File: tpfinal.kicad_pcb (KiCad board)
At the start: 2 copper layers, 108.1 x 81.5 mm, 17 parts, among them J1 220V, J2 1,5-30V 1,5A, SW2 SW_SPST, U1 LM317_TO-220

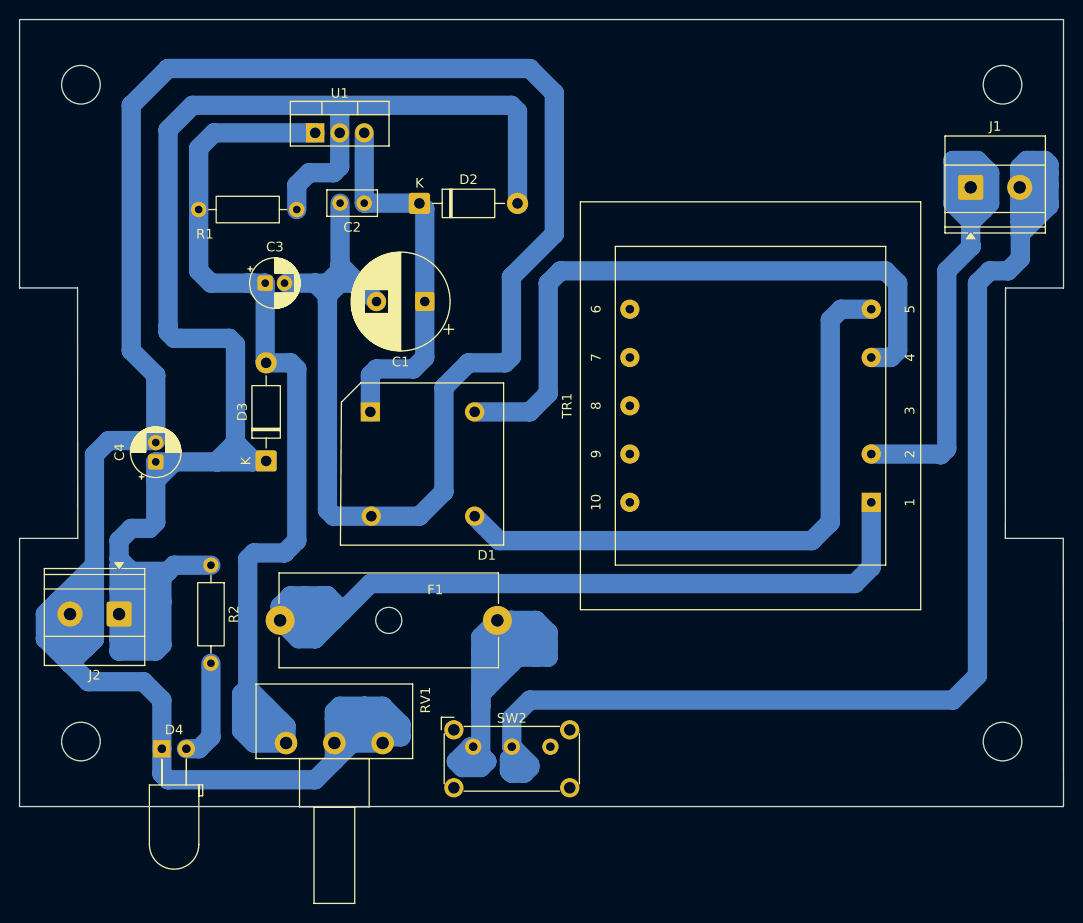
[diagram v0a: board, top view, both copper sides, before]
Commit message: Update
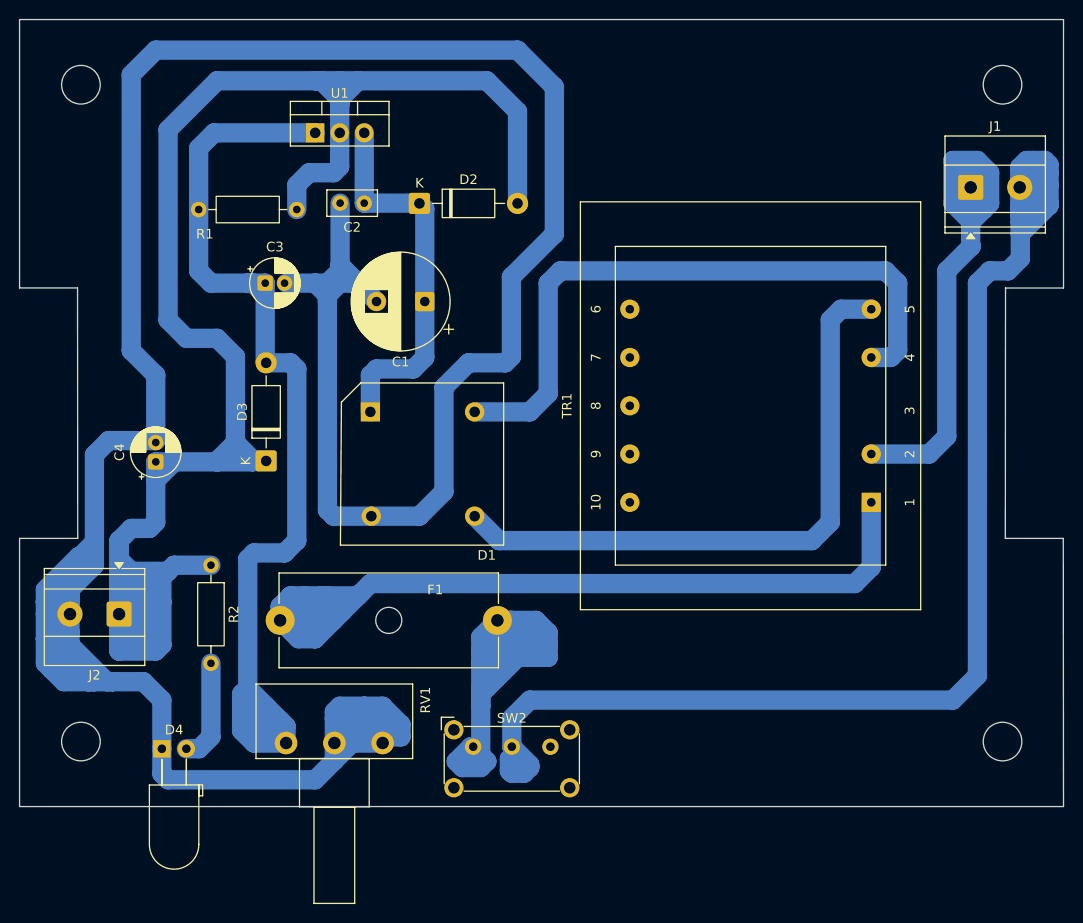
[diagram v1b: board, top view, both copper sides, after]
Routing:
- net +VDC: track 197.6 -> 218.6 mm
- net Net-(SW2-B): track 61.9 -> 74.3 mm
- net GND: track 348.6 -> 359.1 mm
- net Net-(F1-Pad2): track 102.5 -> 106.1 mm
- net Net-(J1-Pin_1): track 56.4 -> 55.6 mm
